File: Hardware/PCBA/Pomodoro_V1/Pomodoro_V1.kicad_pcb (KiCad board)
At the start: 4 copper layers, 78 x 78 mm, 155 parts, among them IC1 LDK120M33R, J1 Conn_01x02_Pin, J10 Conn_01x01_Pin, J2 Conn_01x10_Pin, J3 Conn_01x03_Pin, J4 Conn_01x02_Pin, J5 Conn_01x02_Pin, J6 Conn_01x02_Pin, J7 Conn_01x02_Pin, J8 2171800001, J9 Conn_01x04_Pin, SW1 SW_Push, U1 STM32G071RBTx, U2 LIS2HH12

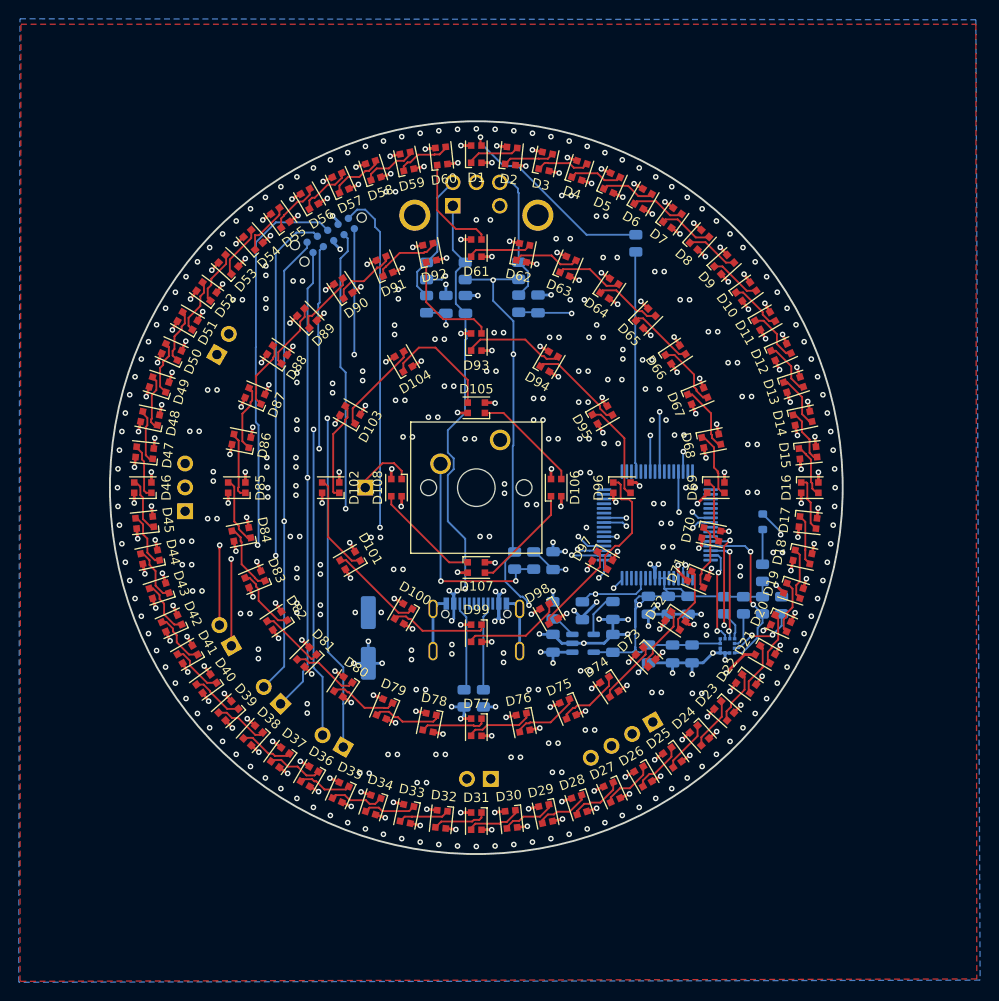
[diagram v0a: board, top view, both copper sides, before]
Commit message: Version that was ordered online
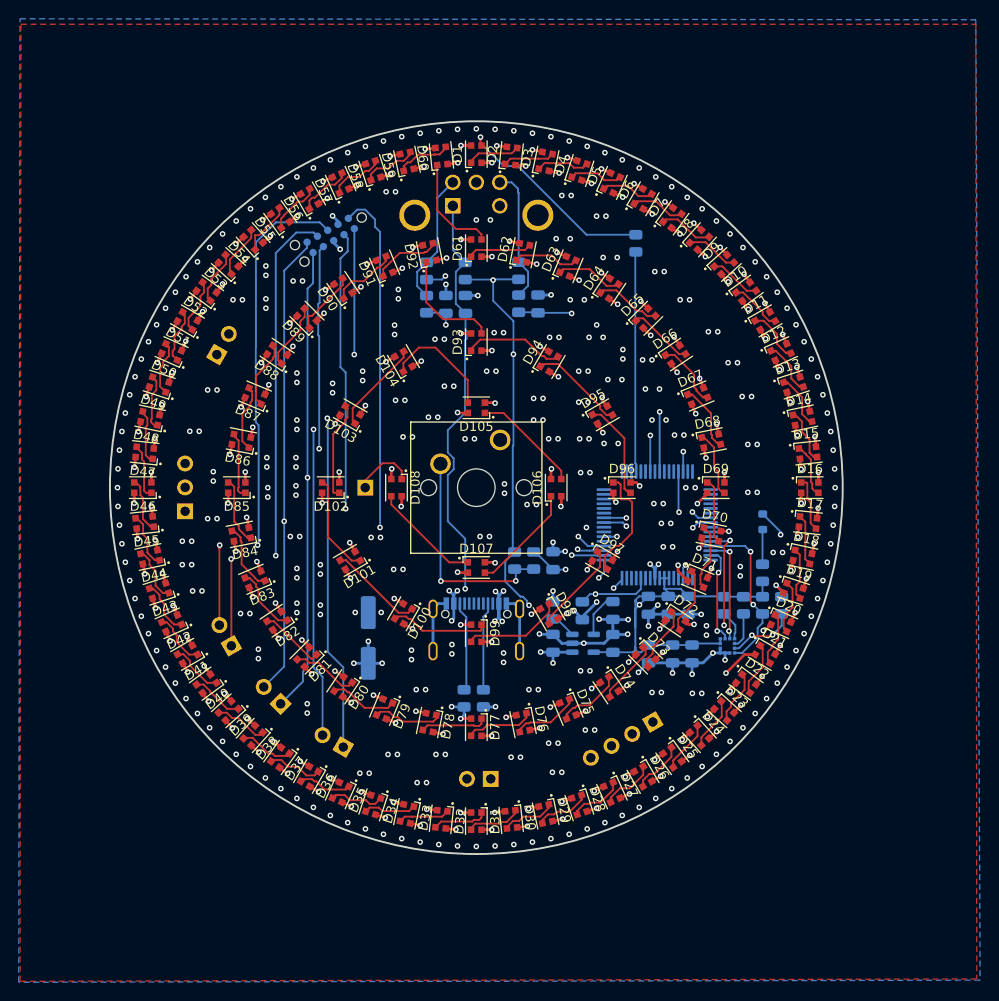
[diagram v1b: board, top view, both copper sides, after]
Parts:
- C15, C18: value 4u7 -> 1u

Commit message: Minor refactoring on the RGBLED Driver, Changed the nominalPomodoro Script a bit, Added some dimensions into Kicad
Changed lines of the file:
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@@
 		)
 		(fp_line
-			(start -1.520001 -1.25)
+			(start -1.520002 -1.25)
 			(end -1.52 1.25)
 			(stroke
@@
 		(fp_line
 			(start -1.52 1.25)
-			(end 1.520001 1.25)
+			(end 1.520002 1.25)
 			(stroke
 				(width 0.05)
@@
 		(fp_line
 			(start 1.52 -1.25)
-			(end -1.520001 -1.25)
+			(end -1.520002 -1.25)
 			(stroke
 				(width 0.05)
@@
 		)
 		(fp_line
-			(start 1.520001 1.25)
+			(start 1.520002 1.25)
 			(end 1.52 -1.25)
 			(stroke
@@
 		)
 		(fp_line
-			(start 1.520001 1.25)
+			(start 1.520002 1.25)
 			(end 1.52 -1.25)
 			(stroke
@@
 		(fp_line
 			(start 1.52 -1.25)
-			(end -1.520001 -1.25)
+			(end -1.520002 -1.25)
 			(stroke
 				(width 0.05)
@@
 		(fp_line
 			(start -1.52 1.25)
-			(end 1.520001 1.25)
+			(end 1.520002 1.25)
 			(stroke
 				(width 0.05)
@@
 		)
 		(fp_line
-			(start -1.520001 -1.25)
+			(start -1.520002 -1.25)
 			(end -1.52 1.25)
 			(stroke
@@
 		(fp_line
 			(start 1.52 -1.25)
-			(end -1.520001 -1.25)
+			(end -1.520002 -1.25)
 			(stroke
 				(width 0.05)
@@
 		)
 		(fp_line
-			(start -1.520001 -1.25)
+			(start -1.520002 -1.25)
 			(end -1.52 1.25)
 			(stroke
@@
 		)
 		(fp_line
-			(start 1.520001 1.25)
+			(start 1.520002 1.25)
 			(end 1.52 -1.25)
 			(stroke
@@
 		(fp_line
 			(start -1.52 1.25)
-			(end 1.520001 1.25)
+			(end 1.520002 1.25)
 			(stroke
 				(width 0.05)
@@
 		(fp_circle
 			(center -1.8 -1)
-			(end -1.7 -1.000001)
+			(end -1.7 -1.000002)
 			(stroke
 				(width 0.1)
@@
 		)
 		(fp_line
-			(start -0.550001 -1)
+			(start -0.550002 -1)
 			(end -1.1 -0.45)
 			(stroke
@@
 		(fp_line
 			(start 1.1 -1)
-			(end -0.550001 -1)
+			(end -0.550002 -1)
 			(stroke
 				(width 0.1)
@@
 		(fp_line
 			(start -1.52 -1.25)
-			(end -1.520001 1.25)
+			(end -1.520002 1.25)
 			(stroke
 				(width 0.05)
@@
 		)
 		(fp_line
-			(start 1.520001 -1.25)
+			(start 1.520002 -1.25)
 			(end -1.52 -1.25)
 			(stroke
@@
 		)
 		(fp_line
-			(start -1.520001 1.25)
+			(start -1.520002 1.25)
 			(end 1.52 1.25)
 			(stroke
@@
 		(fp_line
 			(start 1.52 1.25)
-			(end 1.520001 -1.25)
+			(end 1.520002 -1.25)
 			(stroke
 				(width 0.05)
@@
 		)
 		(fp_line
-			(start 1.520001 -1.25)
+			(start 1.520002 -1.25)
 			(end -1.52 -1.25)
 			(stroke
@@
 		(fp_line
 			(start 1.52 1.25)
-			(end 1.520001 -1.25)
+			(end 1.520002 -1.25)
 			(stroke
 				(width 0.05)
@@
 		(fp_line
 			(start -1.52 -1.25)
-			(end -1.520001 1.25)
+			(end -1.520002 1.25)
 			(stroke
 				(width 0.05)
@@
 		)
 		(fp_line
-			(start -1.520001 1.25)
+			(start -1.520002 1.25)
 			(end 1.52 1.25)
 			(stroke
@@
 		(fp_circle
 			(center -1.8 -1)
-			(end -1.7 -1.000001)
+			(end -1.7 -1.000002)
 			(stroke
 				(width 0.1)
@@
 		(fp_line
 			(start 1.1 -1)
-			(end -0.550001 -1)
+			(end -0.550002 -1)
 			(stroke
 				(width 0.1)
@@
 		)
 		(fp_line
-			(start -0.550001 -1)
+			(start -0.550002 -1)
 			(end -1.1 -0.45)
 			(stroke
@@
 		(fp_line
 			(start 1.52 1.25)
-			(end 1.520001 -1.25)
+			(end 1.520002 -1.25)
 			(stroke
 				(width 0.05)
@@
 		)
 		(fp_line
-			(start -1.520001 1.25)
+			(start -1.520002 1.25)
 			(end 1.52 1.25)
 			(stroke
@@
 		)
 		(fp_line
-			(start 1.520001 -1.25)
+			(start 1.520002 -1.25)
 			(end -1.52 -1.25)
 			(stroke
@@
 		(fp_line
 			(start -1.52 -1.25)
-			(end -1.520001 1.25)
+			(end -1.520002 1.25)
 			(stroke
 				(width 0.05)
@@
 		(fp_line
 			(start -1.52 1.25)
-			(end 1.520001 1.25)
+			(end 1.520002 1.25)
 			(stroke
 				(width 0.05)
@@
 		)
 		(fp_line
-			(start 1.520001 1.25)
+			(start 1.520002 1.25)
 			(end 1.52 -1.25)
 			(stroke
@@
 		)
 		(fp_line
-			(start -1.520001 -1.25)
+			(start -1.520002 -1.25)
 			(end -1.52 1.25)
 			(stroke
@@
 		(fp_line
 			(start 1.52 -1.25)
-			(end -1.520001 -1.25)
+			(end -1.520002 -1.25)
 			(stroke
 				(width 0.05)
@@
 		(fp_circle
 			(center -1.8 -1)
-			(end -1.7 -1.000001)
+			(end -1.7 -1.000002)
 			(stroke
 				(width 0.1)
@@
 		)
 		(fp_line
-			(start -0.550001 -1)
+			(start -0.550002 -1)
 			(end -1.1 -0.45)
 			(stroke
@@
 		(fp_line
 			(start 1.1 -1)
-			(end -0.550001 -1)
+			(end -0.550002 -1)
 			(stroke
 				(width 0.1)
@@
 		(fp_circle
 			(center -1.8 -1)
-			(end -1.7 -1.000001)
+			(end -1.7 -1.000002)
 			(stroke
 				(width 0.1)
@@
 		(fp_line
 			(start 1.1 -1)
-			(end -0.550001 -1)
+			(end -0.550002 -1)
 			(stroke
 				(width 0.1)
@@
 		)
 		(fp_line
-			(start -0.550001 -1)
+			(start -0.550002 -1)
 			(end -1.1 -0.45)
 			(stroke
@@
 		)
 		(fp_line
-			(start -1.520001 1.25)
+			(start -1.520002 1.25)
 			(end 1.52 1.25)
 			(stroke
@@
 		(fp_line
 			(start -1.52 -1.25)
-			(end -1.520001 1.25)
+			(end -1.520002 1.25)
 			(stroke
 				(width 0.05)
@@
 		(fp_line
 			(start 1.52 1.25)
-			(end 1.520001 -1.25)
+			(end 1.520002 -1.25)
 			(stroke
 				(width 0.05)
@@
 		)
 		(fp_line
-			(start 1.520001 -1.25)
+			(start 1.520002 -1.25)
 			(end -1.52 -1.25)
 			(stroke
@@
 		(tags "resistor")
 		(property "Reference" "R13"
-			(at 0 1.65 270)
+			(at 0 1.65 -90)
 			(layer "B.SilkS")
 			(hide yes)
@@
 		)
 		(property "Value" "270"
-			(at 0 -1.65 270)
+			(at 0 -1.65 -90)
 			(layer "B.Fab")
 			(effects
@@
 		)
 		(fp_text user "${REFERENCE}"
-			(at 0 0 270)
+			(at 0 0 -90)
 			(layer "B.Fab")
 			(effects
@@
 		(tags "Through hole pin header THT 1x03 2.54mm single row")
 		(property "Reference" "J3"
-			(at 0 2.33 360)
+			(at 0 2.33 0)
 			(layer "B.SilkS")
 			(hide yes)
@@
 		)
 		(property "Value" "Conn_01x03_Pin"
-			(at 0 -7.41 360)
+			(at 0 -7.41 0)
 			(layer "B.Fab")
 			(hide yes)
@@
 		)
 	)
+	(dimension
+		(type aligned)
+		(layer "Dwgs.User")
+		(pts
+			(xy 139 100) (xy 161 100)
+		)
+		(height -37.33)
+		(gr_text "22.0000 mm"
+			(at 150 61.52 0)
+			(layer "Dwgs.User")
+			(effects
+				(font
+					(size 1 1)
+					(thickness 0.15)
+				)
+			)
+		)
+		(format
+			(prefix "")
+			(suffix "")
+			(units 3)
+			(units_format 1)
+			(precision 4)
+		)
+		(style
+			(thickness 0.1)
+			(arrow_length 1.27)
+			(text_position_mode 0)
+			(extension_height 0.58642)
+			(extension_offset 0.5) keep_text_aligned)
+	)
+	(dimension
+		(type aligned)
+		(layer "Dwgs.User")
+		(pts
+			(xy 109.02 102.58) (xy 191.02 102.58)
+		)
+		(height -50.01)
+		(gr_text "82.0000 mm"
+			(at 150.02 51.42 0)
+			(layer "Dwgs.User")
+			(effects
+				(font
+					(size 1 1)
+					(thickness 0.15)
+				)
+			)
+		)
+		(format
+			(prefix "")
+			(suffix "")
+			(units 3)
+			(units_format 1)
+			(precision 4)
+		)
+		(style
+			(thickness 0.1)
+			(arrow_length 1.27)
+			(text_position_mode 0)
+			(extension_height 0.58642)
+			(extension_offset 0.5) keep_text_aligned)
+	)
+	(dimension
+		(type aligned)
+		(layer "Dwgs.User")
+		(pts
+			(xy 129 100) (xy 171 100)
+		)
+		(height -42.18)
+		(gr_text "42.0000 mm"
+			(at 150 56.67 0)
+			(layer "Dwgs.User")
+			(effects
+				(font
+					(size 1 1)
+					(thickness 0.15)
+				)
+			)
+		)
+		(format
+			(prefix "")
+			(suffix "")
+			(units 3)
+			(units_format 1)
+			(precision 4)
+		)
+		(style
+			(thickness 0.1)
+			(arrow_length 1.27)
+			(text_position_mode 0)
+			(extension_height 0.58642)
+			(extension_offset 0.5) keep_text_aligned)
+	)
+	(dimension
+		(type aligned)
+		(layer "Dwgs.User")
+		(pts
+			(xy 119 99.985) (xy 181 100)
+		)
+		(height -44.443817)
+		(gr_text "62.0000 mm"
+			(at 150.011031 54.398684 359.9861381)
+			(layer "Dwgs.User")
+			(effects
+				(font
+					(size 1 1)
+					(thickness 0.15)
+				)
+			)
+		)
+		(format
+			(prefix "")
+			(suffix "")
+			(units 3)
+			(units_format 1)
+			(precision 4)
+		)
+		(style
+			(thickness 0.1)
+			(arrow_length 1.27)
+			(text_position_mode 0)
+			(extension_height 0.58642)
+			(extension_offset 0.5) keep_text_aligned)
+	)
 	(segment
